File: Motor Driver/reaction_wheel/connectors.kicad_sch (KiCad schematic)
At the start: 6 parts, among them J1 Input Power, J4 Data Conn, J8 MOTOR_OUT

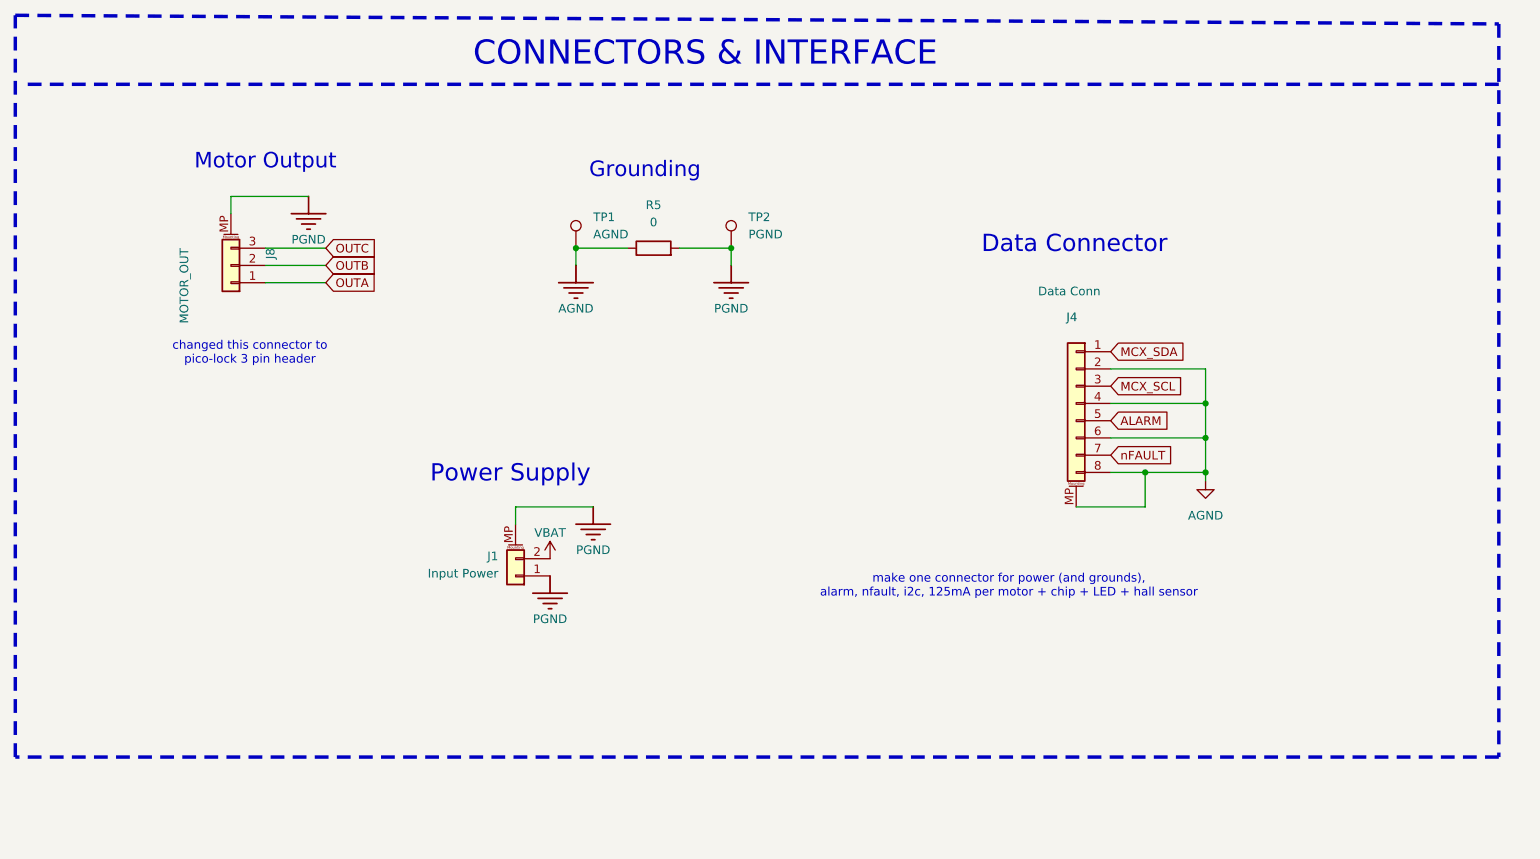
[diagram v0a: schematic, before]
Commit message: Schematic cleanup
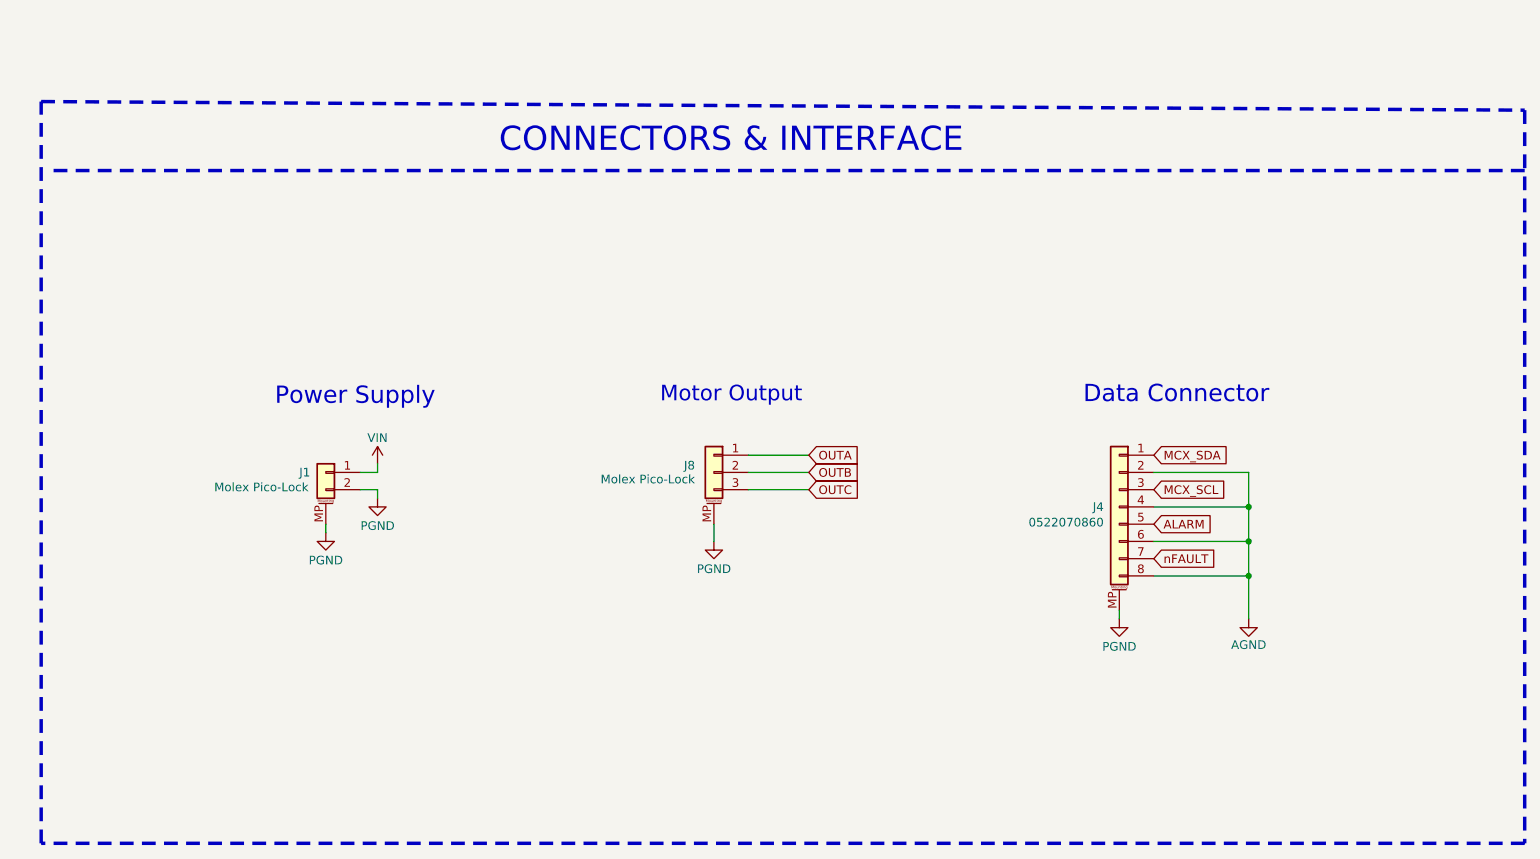
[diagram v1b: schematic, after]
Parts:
- removed R5: 0, Resistor_SMD:R_0603_1608Metric, symbol Device:R
- removed TP1: AGND, TestPoint:TestPoint_Keystone_5000-5004_Miniature, symbol Connector:TestPoint
- removed TP2: PGND, TestPoint:TestPoint_Keystone_5000-5004_Miniature, symbol Connector:TestPoint
- J1: value Input Power -> Molex Pico-Lock
- J4: value Data Conn -> 0522070860
- J8: value MOTOR_OUT -> Molex Pico-Lock
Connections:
- net VBAT is gone; now on net PGND: J1.2 (Pin_2)
- net AGND: no longer J4.MP (MountPin)
- net PGND: now also J4.MP (MountPin); no longer J1.1 (Pin_1)
- new net VIN: J1.1 (Pin_1)
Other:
- note removed: "Grounding"
- note removed: "changed this connector to pico-lock 3 pin header"
- note removed: "make one connector for power (and grounds), alarm, nfault, i2c, 125mA per motor + chip + LED + hall sensor"
- moved on the sheet: J1, J4, J8
